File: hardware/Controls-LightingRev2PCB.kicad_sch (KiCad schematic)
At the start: 34 parts, among them IC3 ACS724LLCTR-05AU-T, IC4 ACS724LLCTR-05AU-T, IC5 TLV70433DBVT, IC6 ACS724LLCTR-05AU-T, J1 53307-2471, J2 MX150_02x08_RightAngle, J3 Conn_02x05_Top_Bottom, J4 Conn_01x02, J5 Conn_01x02, J6 Conn_01x03, Q3 IRLML0030, Q5 IRLML0030, U5 SN74LV1T34DBV

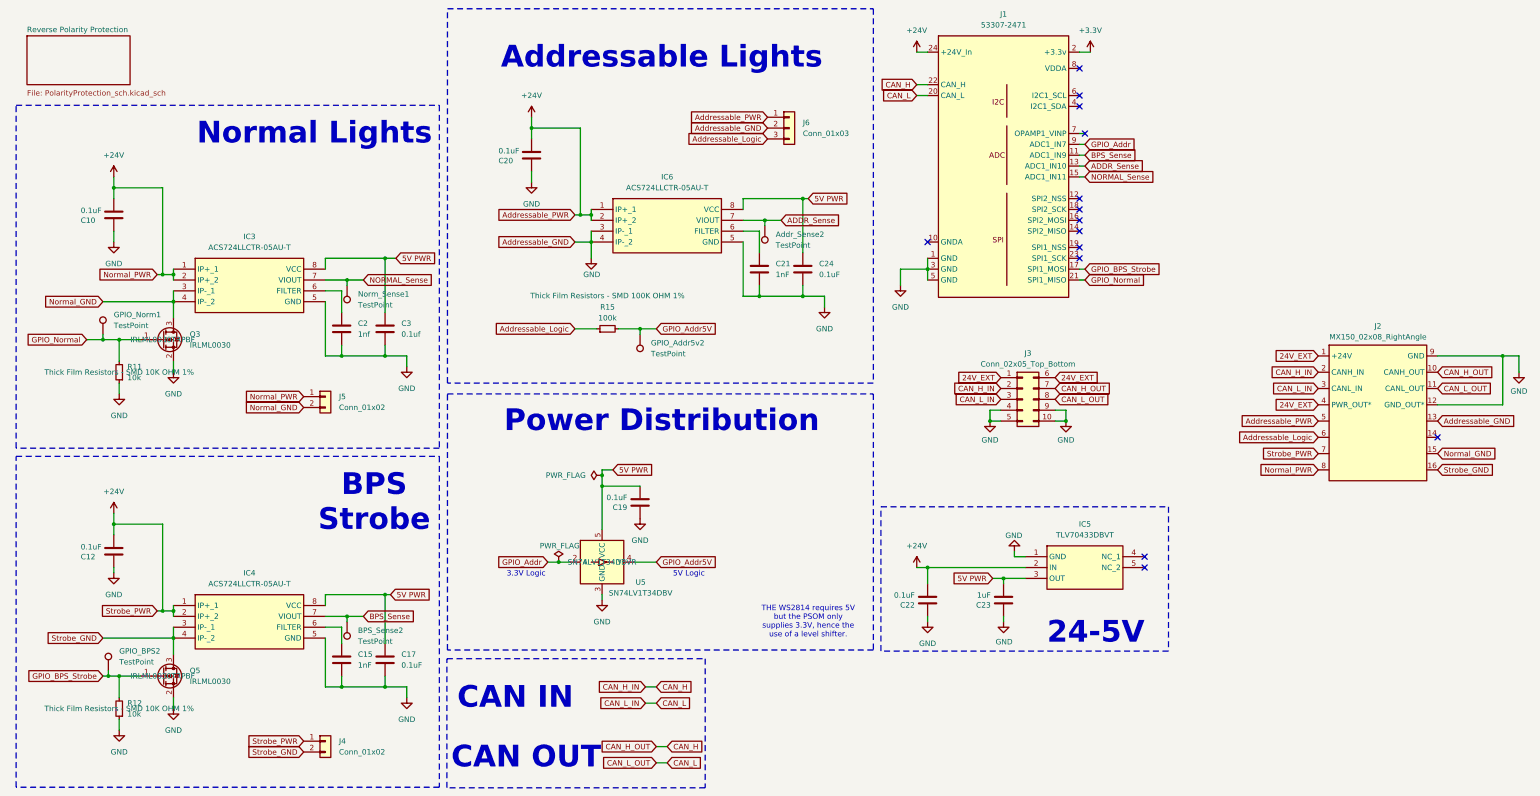
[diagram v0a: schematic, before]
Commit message: Current Layout
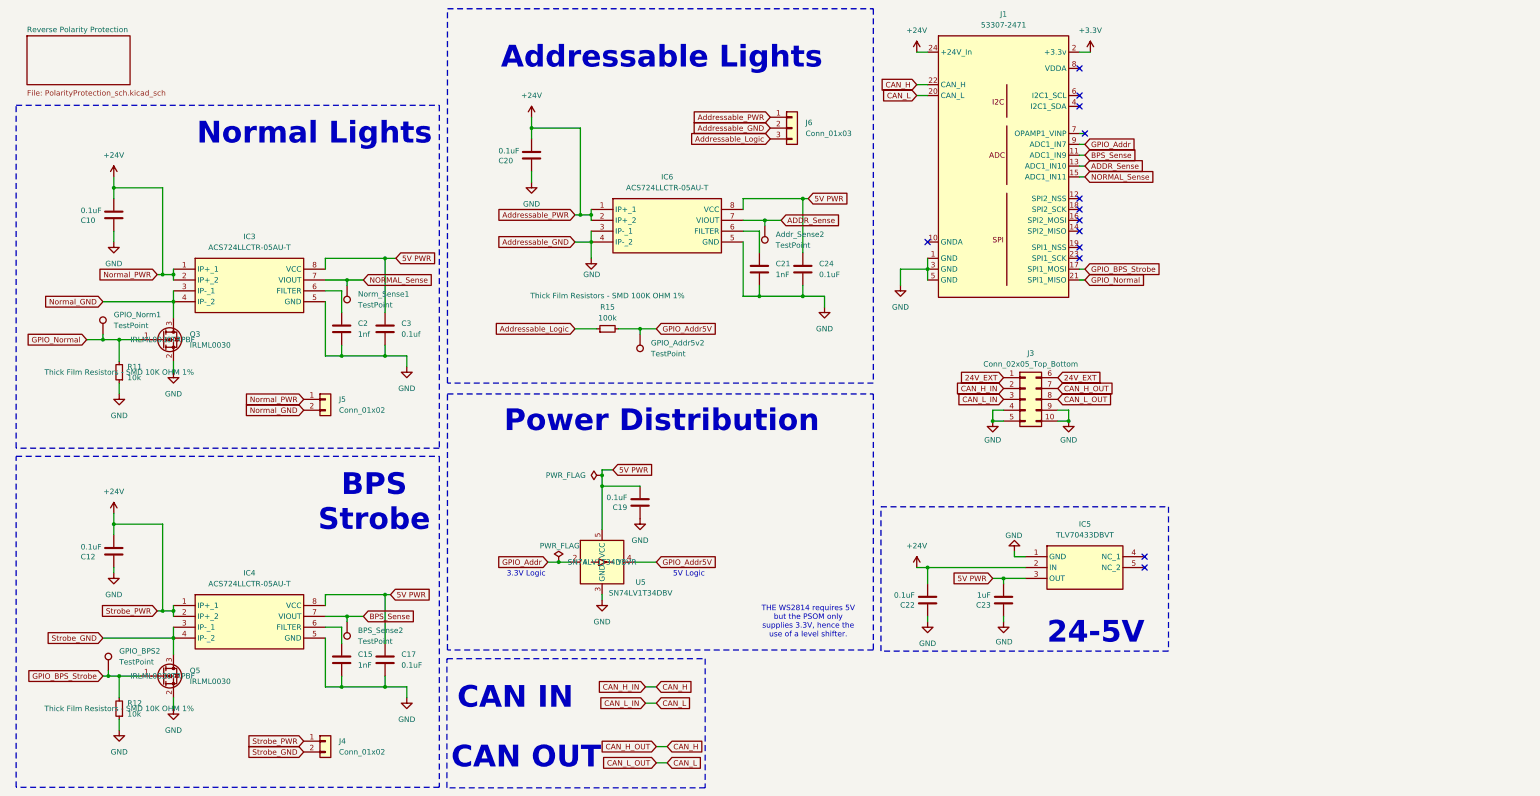
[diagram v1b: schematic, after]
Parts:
- removed J2: MX150_02x08_RightAngle, UTSVT_Connectors:MX150_02x08_RightAngle, symbol UTSVT-Connectors:MX150_02x08_RightAngle
- J3: footprint (none) -> Connector_Molex:Molex_Nano-Fit_105314-xx10_2x05_P2.50mm_Horizontal
- J4, J5: footprint (none) -> UTSVT_Connectors:105313-2102
- J6: footprint (none) -> UTSVT_Connectors:105313-1103
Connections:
- no-connect marks 14 -> 13
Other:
- moved on the sheet: J3, J5, J6

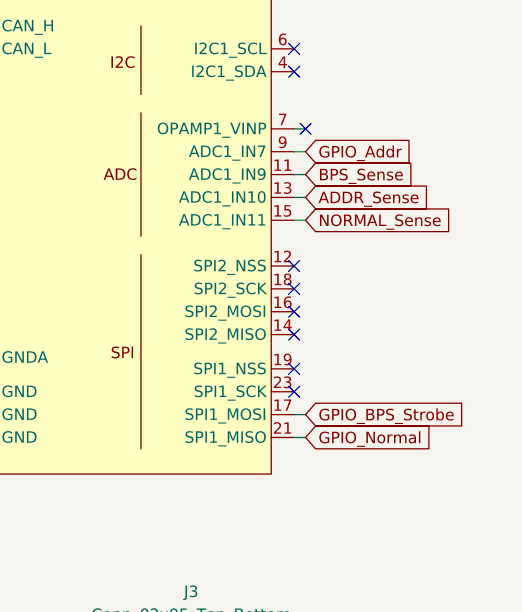
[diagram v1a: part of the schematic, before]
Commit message: Layout
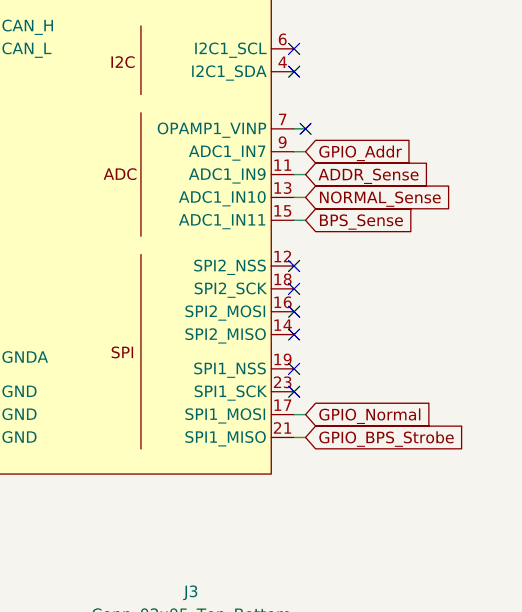
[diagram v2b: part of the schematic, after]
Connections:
- net ADDR_Sense: now also J1.11 (ADC1_IN9); no longer J1.13 (ADC1_IN10)
- net BPS_Sense: now also J1.15 (ADC1_IN11); no longer J1.11 (ADC1_IN9)
- net GPIO_BPS_Strobe: now also J1.21 (SPI1_MISO); no longer J1.17 (SPI1_MOSI)
- net GPIO_Normal: now also J1.17 (SPI1_MOSI); no longer J1.21 (SPI1_MISO)
- net NORMAL_Sense: now also J1.13 (ADC1_IN10); no longer J1.15 (ADC1_IN11)

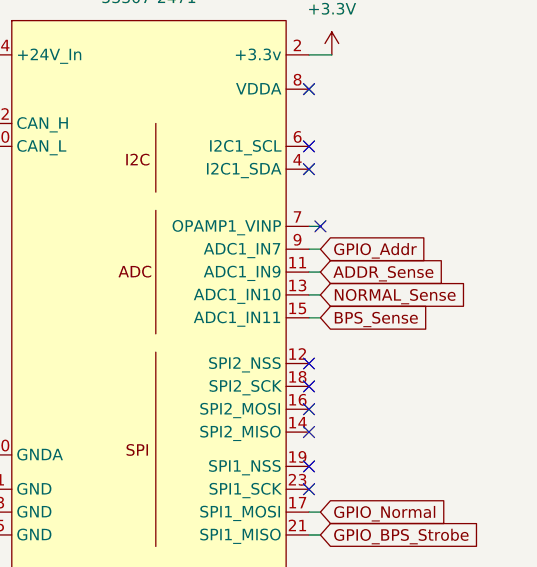
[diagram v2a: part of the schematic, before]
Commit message: Layout Review
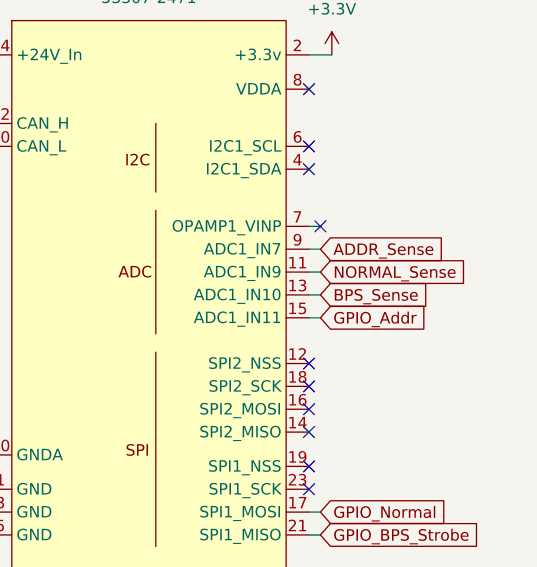
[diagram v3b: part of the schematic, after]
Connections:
- net ADDR_Sense: now also J1.9 (ADC1_IN7); no longer J1.11 (ADC1_IN9)
- net BPS_Sense: now also J1.13 (ADC1_IN10); no longer J1.15 (ADC1_IN11)
- net GPIO_Addr: now also J1.15 (ADC1_IN11); no longer J1.9 (ADC1_IN7)
- net NORMAL_Sense: now also J1.11 (ADC1_IN9); no longer J1.13 (ADC1_IN10)

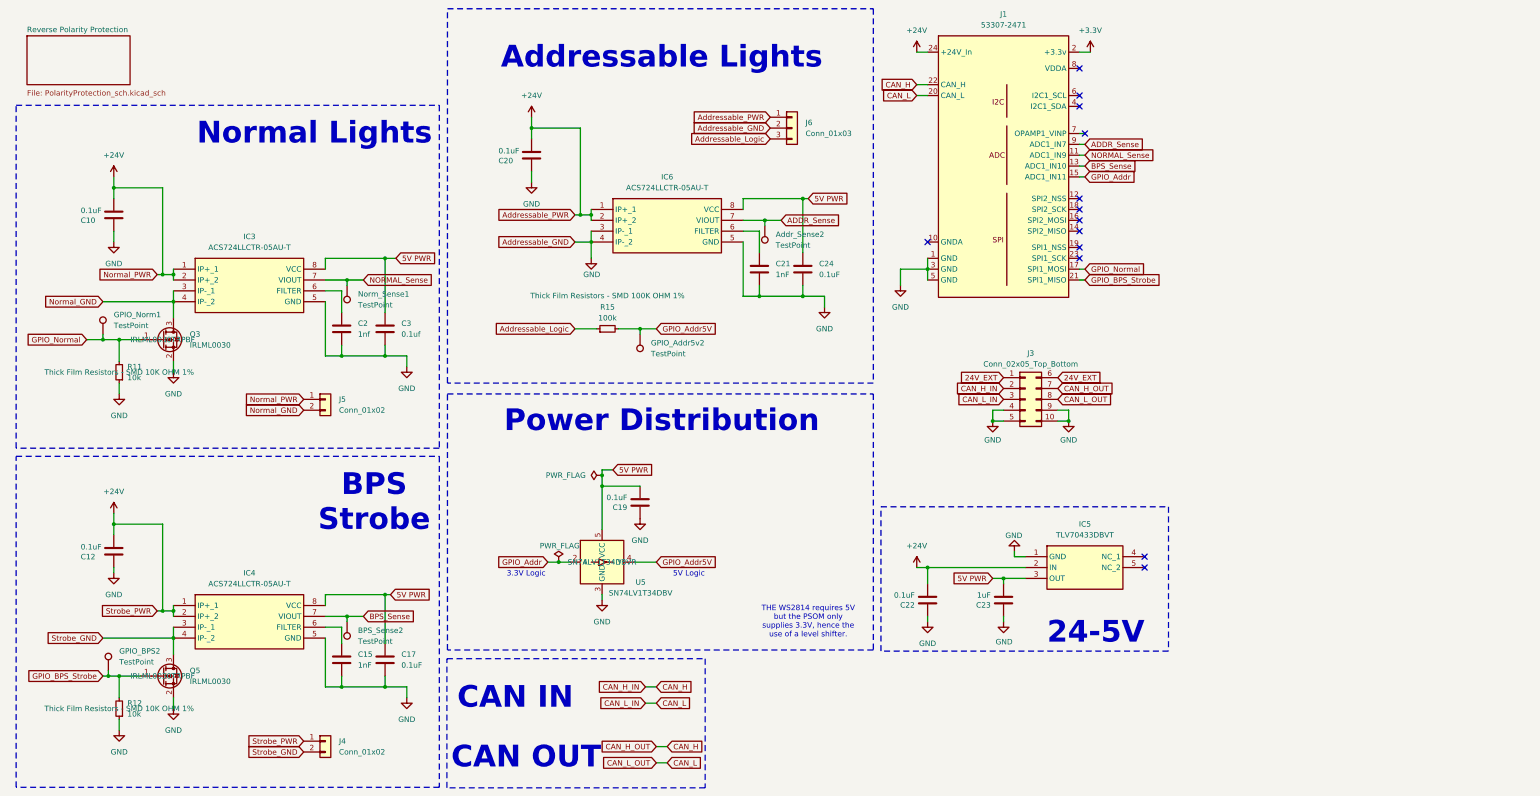
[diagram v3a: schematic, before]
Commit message: Some routing
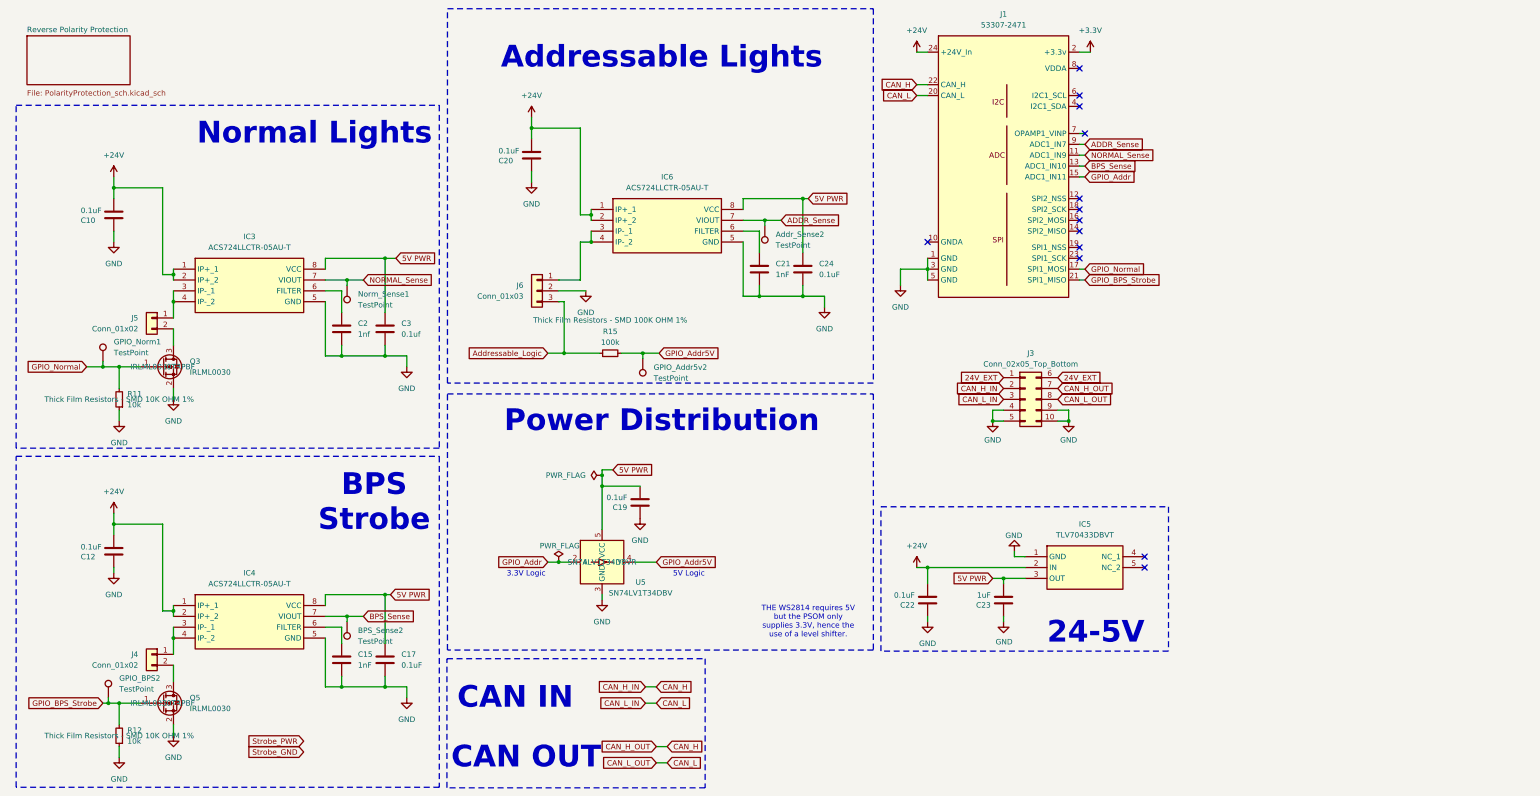
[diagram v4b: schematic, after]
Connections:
- net +24V: no longer J4.1 (Pin_1), J5.1 (Pin_1), J6.1 (Pin_1)
- net GND: no longer IC6.3 (IP-_1), IC6.4 (IP-_2)
- net Strobe_GND: no longer IC4.3 (IP-_1), IC4.4 (IP-_2), J4.2 (Pin_2), Q5.3 (D)
- net Normal_GND: no longer names the net of IC3.3 (IP-_1), IC3.4 (IP-_2)
- net Normal_GND: now also J5.1 (Pin_1); no longer J5.2 (Pin_2), Q3.3 (D)
- new net: IC6.3 (IP-_1), IC6.4 (IP-_2), J6.1 (Pin_1)
- new net: IC4.3 (IP-_1), IC4.4 (IP-_2), J4.1 (Pin_1)
- new net: J4.2 (Pin_2), Q5.3 (D)
- new net: J5.2 (Pin_2), Q3.3 (D)
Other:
- moved on the sheet: GPIO_Addr5v2, GPIO_BPS2, GPIO_Norm1, J4, J5, J6, Q3, Q5, R11, R12, R15
